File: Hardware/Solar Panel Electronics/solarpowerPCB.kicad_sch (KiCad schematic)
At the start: 41 parts, among them J3 Conn_01x02_Male, J4 Conn_01x06_Male, J5 Conn_01x02_Male, Q1 MMDT2222A, U1 SN65HVD230, U2 ESP32-WROOM-32D

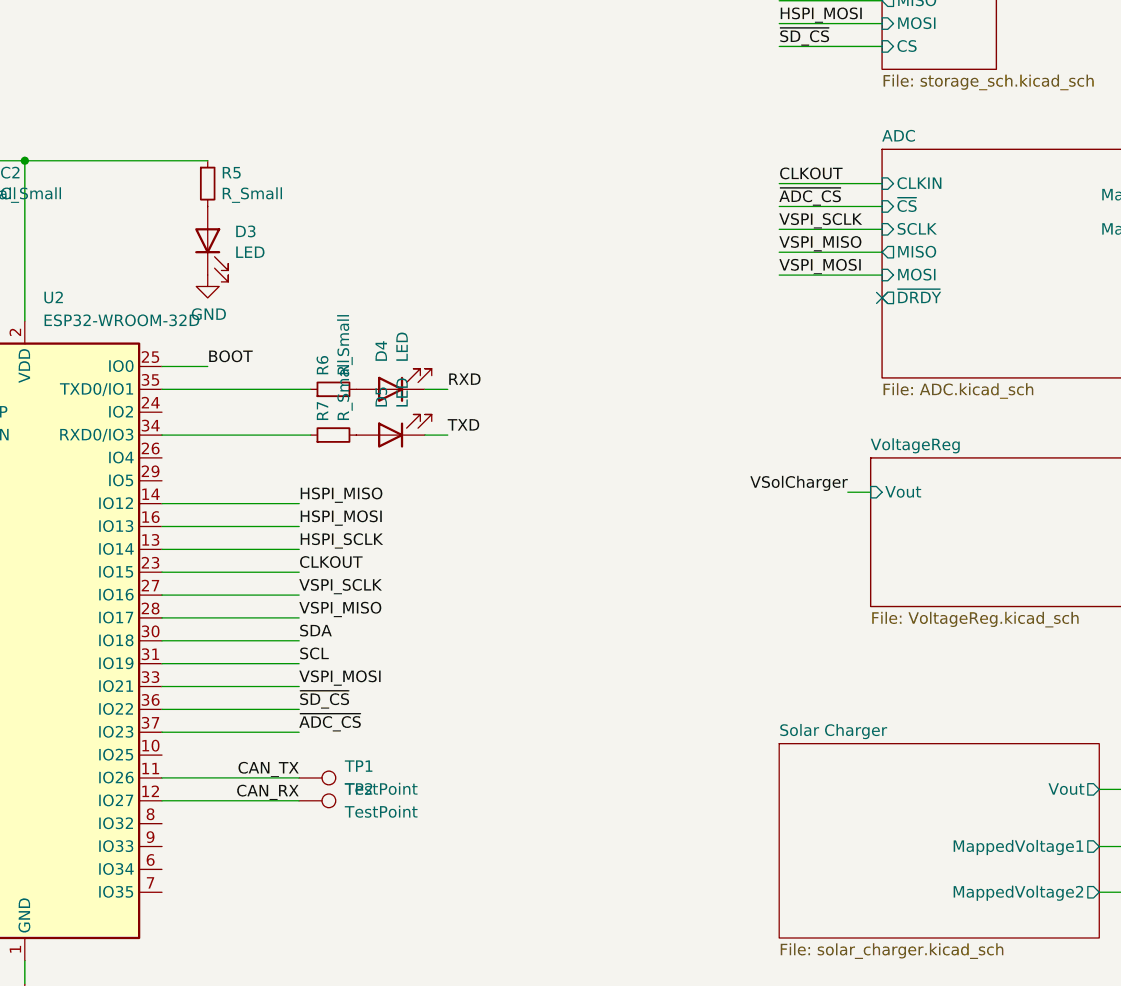
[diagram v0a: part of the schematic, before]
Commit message: ICARUS v2
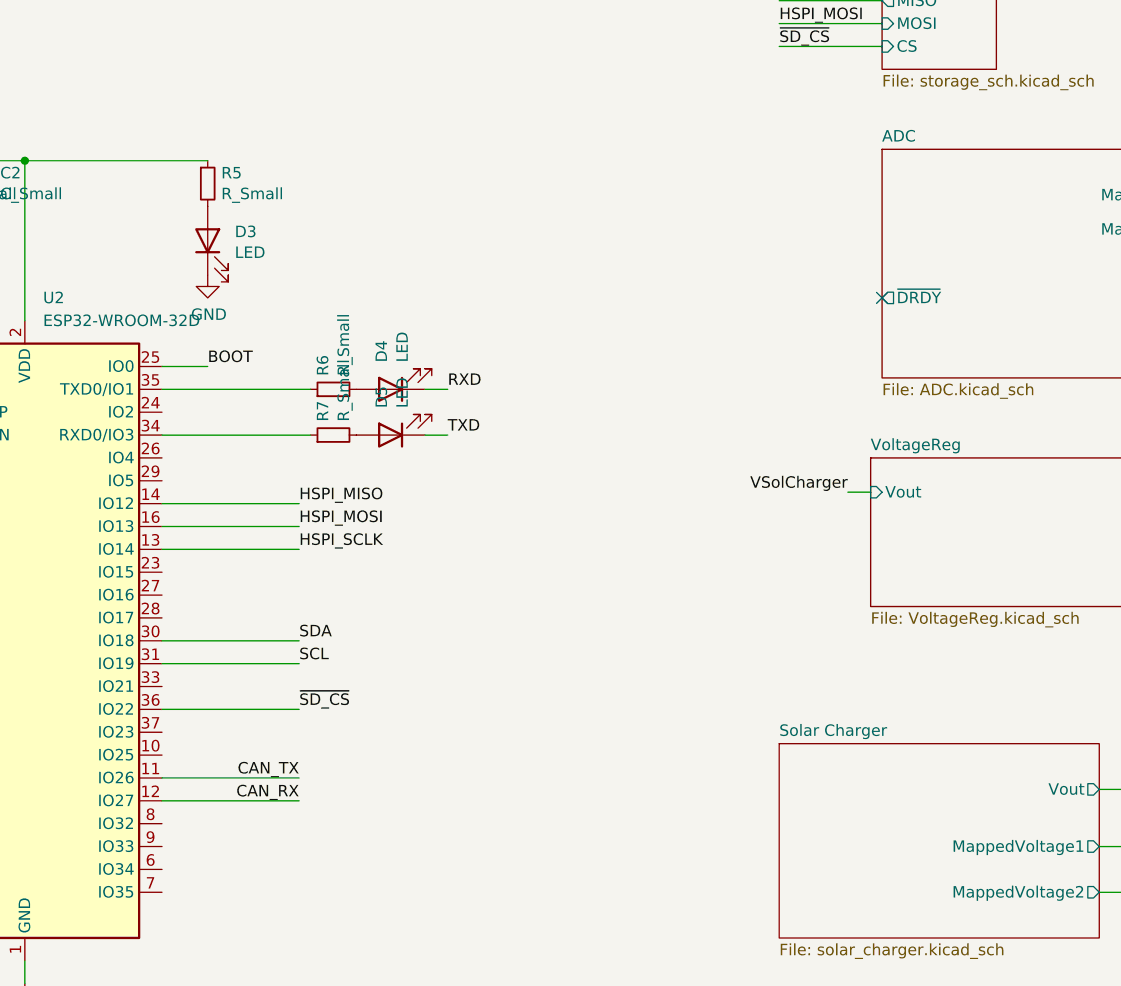
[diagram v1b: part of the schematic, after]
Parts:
- removed TP1, TP2: TestPoint, TestPoint:TestPoint_Pad_D1.0mm, symbol Connector:TestPoint
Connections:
- net CLKOUT: no longer names the net of U2.23 (IO15)
- net VSPI_MISO: no longer names the net of U2.28 (IO17)
- net VSPI_MOSI: no longer names the net of U2.33 (IO21)
- net VSPI_SCLK: no longer names the net of U2.27 (IO16)
- net ~{ADC_CS}: no longer names the net of U2.37 (IO23)
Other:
- sheet ADC ports: added none; removed CLKIN, MISO, MOSI, SCLK, ~{CS}
